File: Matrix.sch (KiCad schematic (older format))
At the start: 216 parts

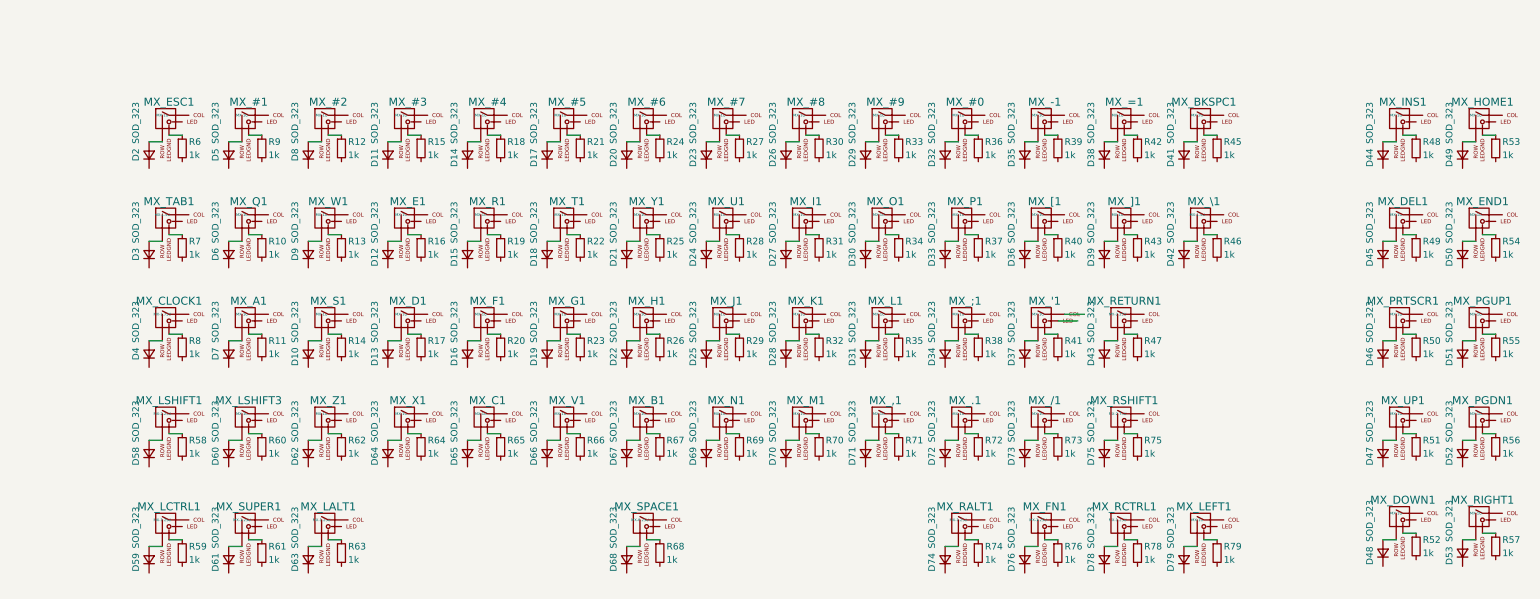
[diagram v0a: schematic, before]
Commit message: Position switch matrix
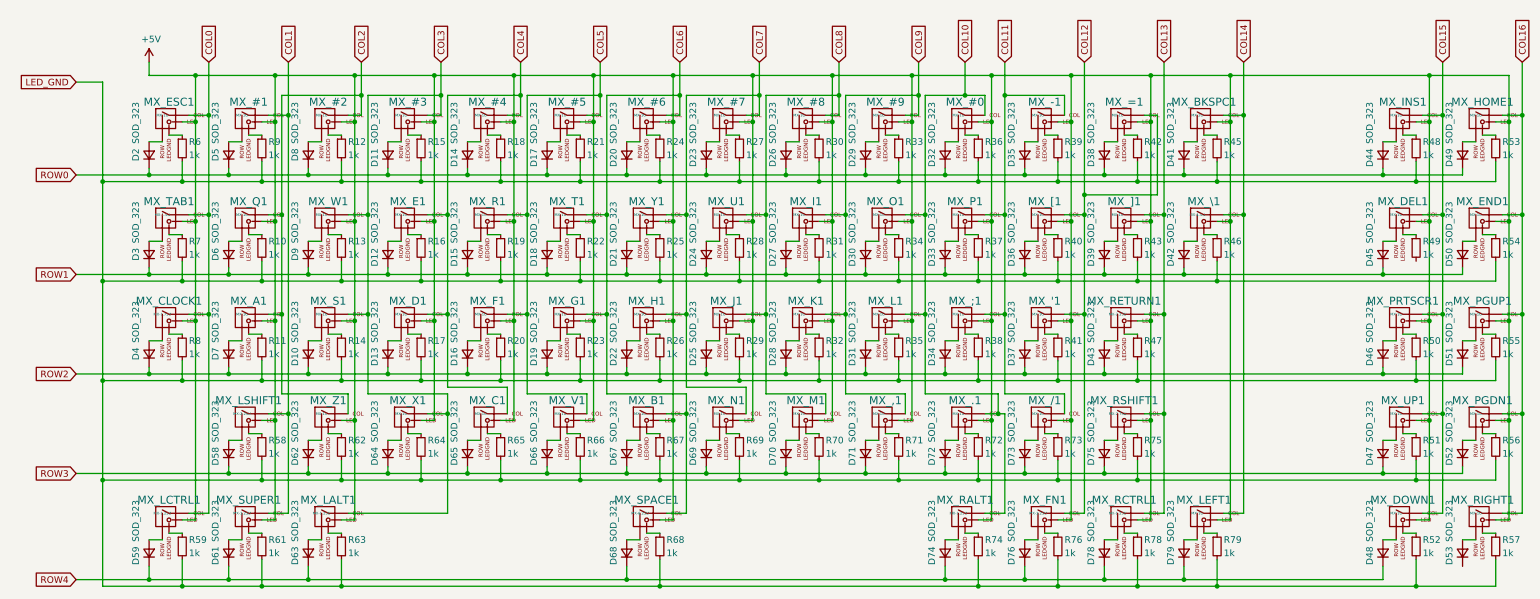
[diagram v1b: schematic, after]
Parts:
- removed D60: SOD_323, symbol Device:D_Small
- removed MX_LSHIFT3: MX-1U, symbol MX_Alps_Hybrid:MX-LED
- removed R60: 1k, symbol Device:R_Small
- D10, D11, D12, D13, D14, D15, D16, D17, D18, D19, D2, D20, D21, D22, D23, D24, D25, D26, D27, D28, D29, D3, D30, D31, D32, D33, D34, D35, D36, D37, D38, D39, D4, D41, D42, D43, D44, D45, D46, D47, D48, D49, D5, D50, D51, D52, D53, D58, D59, D6, D61, D62, D63, D64, D65, D66, D67, D68, D69, D7, D70, D71, D72, D73, D74, D75, D76, D78, D79, D8, D9: footprint (none) -> Diode_SMD:D_SOD-323_HandSoldering
- MX_#0, MX_#1, MX_#2, MX_#3, MX_#4, MX_#5, MX_#6, MX_#7, MX_#8, MX_#9, MX_'1, MX_,1, MX_-1, MX_.1, MX_/1, MX_;1, MX_=1, MX_A1, MX_B1, MX_C1, MX_D1, MX_DEL1, MX_DOWN1, MX_E1, MX_END1, MX_ESC1, MX_F1, MX_G1, MX_H1, MX_HOME1, MX_I1, MX_INS1, MX_J1, MX_K1, MX_L1, MX_LEFT1, MX_M1, MX_N1, MX_O1, MX_P1, MX_PGDN1, MX_PGUP1, MX_PRTSCR1, MX_Q1, MX_R1, MX_RIGHT1, MX_S1, MX_T1, MX_U1, MX_UP1, MX_V1, MX_W1, MX_X1, MX_Y1, MX_Z1, MX_[1, MX_]1: footprint (none) -> MX_Alps_Hybrid:MX-1U
- MX_BKSPC1: footprint (none) -> MX_Alps_Hybrid:MX-2U
- MX_CLOCK1: footprint (none) -> MX_Alps_Hybrid:MX-1.75U
- MX_FN1, MX_LALT1, MX_LCTRL1, MX_RALT1, MX_RCTRL1, MX_SUPER1: footprint (none) -> MX_Alps_Hybrid:MX-1.25U
- MX_LSHIFT1, MX_RETURN1: footprint (none) -> MX_Alps_Hybrid:MX-2.25U
- MX_RSHIFT1: footprint (none) -> MX_Alps_Hybrid:MX-2.75U
- MX_SPACE1: footprint (none) -> MX_Alps_Hybrid:MX-6.25U
- MX_TAB1, MX_\1: footprint (none) -> MX_Alps_Hybrid:MX-1.5U
- R10, R11, R12, R13, R14, R15, R16, R17, R18, R19, R20, R21, R22, R23, R24, R25, R26, R27, R28, R29, R30, R31, R32, R33, R34, R35, R36, R37, R38, R39, R40, R41, R42, R43, R45, R46, R47, R48, R49, R50, R51, R52, R53, R54, R55, R56, R57, R58, R59, R6, R61, R62, R63, R64, R65, R66, R67, R68, R69, R7, R70, R71, R72, R73, R74, R75, R76, R78, R79, R8, R9: footprint (none) -> Resistor_SMD:R_0805_2012Metric_Pad1.15x1.40mm_HandSolder
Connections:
- net COL0: now reaches MX_ESC1.1 (COL)
- net COL0: now also MX_CLOCK1.1 (COL), MX_LCTRL1.1 (COL), MX_TAB1.1 (COL)
- net +5V: now reaches MX_ESC1.3 (LED)
- net +5V: now also MX_#0.3 (LED), MX_#1.3 (LED), MX_#2.3 (LED), MX_#3.3 (LED), MX_#4.3 (LED), MX_#5.3 (LED), MX_#6.3 (LED), MX_#7.3 (LED), MX_#8.3 (LED), MX_#9.3 (LED), MX_'1.3 (LED), MX_,1.3 (LED), MX_-1.3 (LED), MX_.1.3 (LED), MX_/1.3 (LED), MX_;1.3 (LED), MX_=1.3 (LED), MX_A1.3 (LED), MX_B1.3 (LED), MX_BKSPC1.3 (LED), MX_C1.3 (LED), MX_CLOCK1.3 (LED), MX_D1.3 (LED), MX_DEL1.3 (LED), MX_DOWN1.3 (LED), MX_E1.3 (LED), MX_END1.3 (LED), MX_F1.3 (LED), MX_FN1.3 (LED), MX_G1.3 (LED), MX_H1.3 (LED), MX_HOME1.3 (LED), MX_I1.3 (LED), MX_INS1.3 (LED), MX_J1.3 (LED), MX_K1.3 (LED), MX_L1.3 (LED), MX_LALT1.3 (LED), MX_LCTRL1.3 (LED), MX_LEFT1.3 (LED), MX_LSHIFT1.3 (LED), MX_M1.3 (LED), MX_N1.3 (LED), MX_O1.3 (LED), MX_P1.3 (LED), MX_PGDN1.3 (LED), MX_PGUP1.3 (LED), MX_PRTSCR1.3 (LED), MX_Q1.3 (LED), MX_R1.3 (LED), MX_RALT1.3 (LED), MX_RCTRL1.3 (LED), MX_RETURN1.3 (LED), MX_RIGHT1.3 (LED), MX_RSHIFT1.3 (LED), MX_S1.3 (LED), MX_SPACE1.3 (LED), MX_SUPER1.3 (LED), MX_T1.3 (LED), MX_TAB1.3 (LED), MX_U1.3 (LED), MX_UP1.3 (LED), MX_V1.3 (LED), MX_W1.3 (LED), MX_X1.3 (LED), MX_Y1.3 (LED), MX_Z1.3 (LED), MX_[1.3 (LED), MX_\1.3 (LED), MX_]1.3 (LED)
- net ROW0: now reaches D2.1 (K)
- net ROW0: now also D11.1 (K), D14.1 (K), D17.1 (K), D20.1 (K), D23.1 (K), D26.1 (K), D29.1 (K), D32.1 (K), D35.1 (K), D38.1 (K), D41.1 (K), D44.1 (K), D49.1 (K), D5.1 (K), D8.1 (K)
- net LED_GND: now reaches R6.2
- net LED_GND: now also R10.2, R11.2, R12.2, R13.2, R14.2, R15.2, R16.2, R17.2, R18.2, R19.2, R20.2, R21.2, R22.2, R23.2, R24.2, R25.2, R26.2, R27.2, R28.2, R29.2, R30.2, R31.2, R32.2, R33.2, R34.2, R35.2, R36.2, R37.2, R38.2, R39.2, R40.2, R41.2, R42.2, R43.2, R45.2, R46.2, R47.2, R48.2, R50.2, R51.2, R52.2, R53.2, R54.2, R55.2, R56.2, R57.2, R58.2, R59.2, R61.2, R62.2, R63.2, R64.2, R65.2, R66.2, R67.2, R68.2, R69.2, R7.2, R70.2, R71.2, R72.2, R73.2, R74.2, R75.2, R76.2, R78.2, R79.2, R8.2, R9.2
- net COL1: now reaches MX_#1.1 (COL)
- net COL1: now also MX_LSHIFT1.1 (COL), MX_SUPER1.1 (COL)
- net COL2: now reaches MX_#2.1 (COL)
- net COL2: now also MX_A1.1 (COL), MX_Q1.1 (COL), MX_Z1.1 (COL)
- net COL3: now reaches MX_#3.1 (COL)
- net COL3: now also MX_LALT1.1 (COL), MX_S1.1 (COL), MX_W1.1 (COL), MX_X1.1 (COL)
- net COL4: now reaches MX_#4.1 (COL)
- net COL4: now also MX_C1.1 (COL), MX_D1.1 (COL), MX_E1.1 (COL)
- net COL5: now reaches MX_#5.1 (COL)
- net COL5: now also MX_F1.1 (COL), MX_R1.1 (COL), MX_V1.1 (COL)
- net COL6: now reaches MX_#6.1 (COL)
- net COL6: now also MX_B1.1 (COL), MX_G1.1 (COL), MX_SPACE1.1 (COL), MX_T1.1 (COL)
- net COL7: now reaches MX_#7.1 (COL)
- net COL7: now also MX_H1.1 (COL), MX_N1.1 (COL), MX_Y1.1 (COL)
- net COL8: now reaches MX_#8.1 (COL)
- net COL8: now also MX_J1.1 (COL), MX_M1.1 (COL), MX_U1.1 (COL)
- net COL9: now reaches MX_#9.1 (COL)
- net COL9: now also MX_,1.1 (COL), MX_I1.1 (COL), MX_K1.1 (COL)
- net COL10: now reaches MX_#0.1 (COL)
- net COL10: now also MX_.1.1 (COL), MX_L1.1 (COL), MX_O1.1 (COL), MX_RALT1.1 (COL)
- net COL11: now reaches MX_-1.1 (COL)
- net COL11: now also MX_/1.1 (COL), MX_;1.1 (COL), MX_P1.1 (COL)
- net COL12: now reaches MX_=1.1 (COL)
- net COL12: now also MX_'1.1 (COL), MX_FN1.1 (COL), MX_[1.1 (COL)
- net COL14: now reaches MX_BKSPC1.1 (COL)
- net COL14: now also MX_LEFT1.1 (COL), MX_\1.1 (COL)
- net ROW3: now reaches D58.1 (K)
- net ROW3: now also D47.1 (K), D52.1 (K), D62.1 (K), D64.1 (K), D65.1 (K), D66.1 (K), D67.1 (K), D69.1 (K), D70.1 (K), D71.1 (K), D72.1 (K), D73.1 (K), D75.1 (K)
- net COL13: now reaches MX_RSHIFT1.1 (COL)
- net COL13: now also MX_RCTRL1.1 (COL), MX_RETURN1.1 (COL), MX_]1.1 (COL)
- net ROW1: now reaches D3.1 (K)
- net ROW1: now also D12.1 (K), D15.1 (K), D18.1 (K), D21.1 (K), D24.1 (K), D27.1 (K), D30.1 (K), D33.1 (K), D36.1 (K), D39.1 (K), D42.1 (K), D45.1 (K), D50.1 (K), D6.1 (K), D9.1 (K)
- net COL15: now reaches MX_INS1.1 (COL)
- net COL15: now also MX_DEL1.1 (COL), MX_DOWN1.1 (COL), MX_PRTSCR1.1 (COL), MX_UP1.1 (COL)
- net COL16: now reaches MX_HOME1.1 (COL)
- net COL16: now also MX_END1.1 (COL), MX_PGDN1.1 (COL), MX_PGUP1.1 (COL), MX_RIGHT1.1 (COL)
- net ROW2: now reaches D46.1 (K)
- net ROW2: now also D10.1 (K), D13.1 (K), D16.1 (K), D19.1 (K), D22.1 (K), D25.1 (K), D28.1 (K), D31.1 (K), D34.1 (K), D37.1 (K), D4.1 (K), D43.1 (K), D51.1 (K), D7.1 (K)
- net ROW4: now reaches D48.1 (K)
- net ROW4: now also D59.1 (K), D61.1 (K), D63.1 (K), D68.1 (K), D74.1 (K), D76.1 (K), D78.1 (K), D79.1 (K)
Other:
- moved on the sheet: D58, D59, D61, D63, D68, D74, D76, D78, D79, MX_FN1, MX_LALT1, MX_LCTRL1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
